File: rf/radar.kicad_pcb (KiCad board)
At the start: 4 copper layers, 52 x 68 mm, 136 parts, among them J101 Conn_01x02, J102 Conn_Coaxial, J103 Conn_01x04, J104 Conn_01x01, J105 Conn_01x01, J106 Conn_Coaxial, J107 Conn_01x02, J108 Conn_01x02, J801 Conn_01x02, T401 2450BL15B100, T402 2450BL15B050, U101 CP0402Q5425ENTR, U201 MAX2750, U202 MC2016K30.0000C16ESH, U203 ADF4153A, U301 QPA5219, U401 AD8343, U501 MGA-645T6, U502 MGA-645T6, U601 TLV4172, U701 SN74LV1T34, U702 SN74LV1T34, U801 ADP150AUJZ-1.8-R7, U802 LM340MPX-5.0/NOPB, U803 L78L33ABU, U804 TPS54308

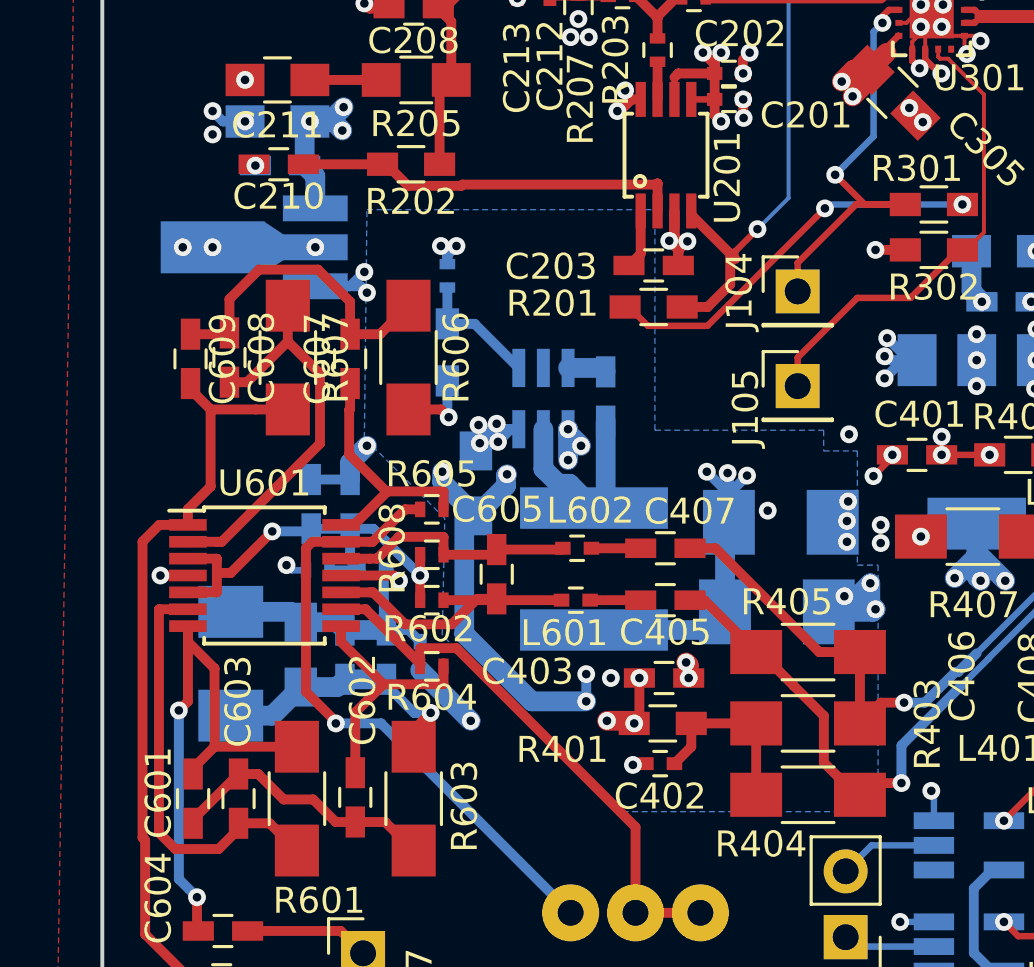
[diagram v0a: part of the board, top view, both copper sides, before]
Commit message: Small fixes; update Gerber
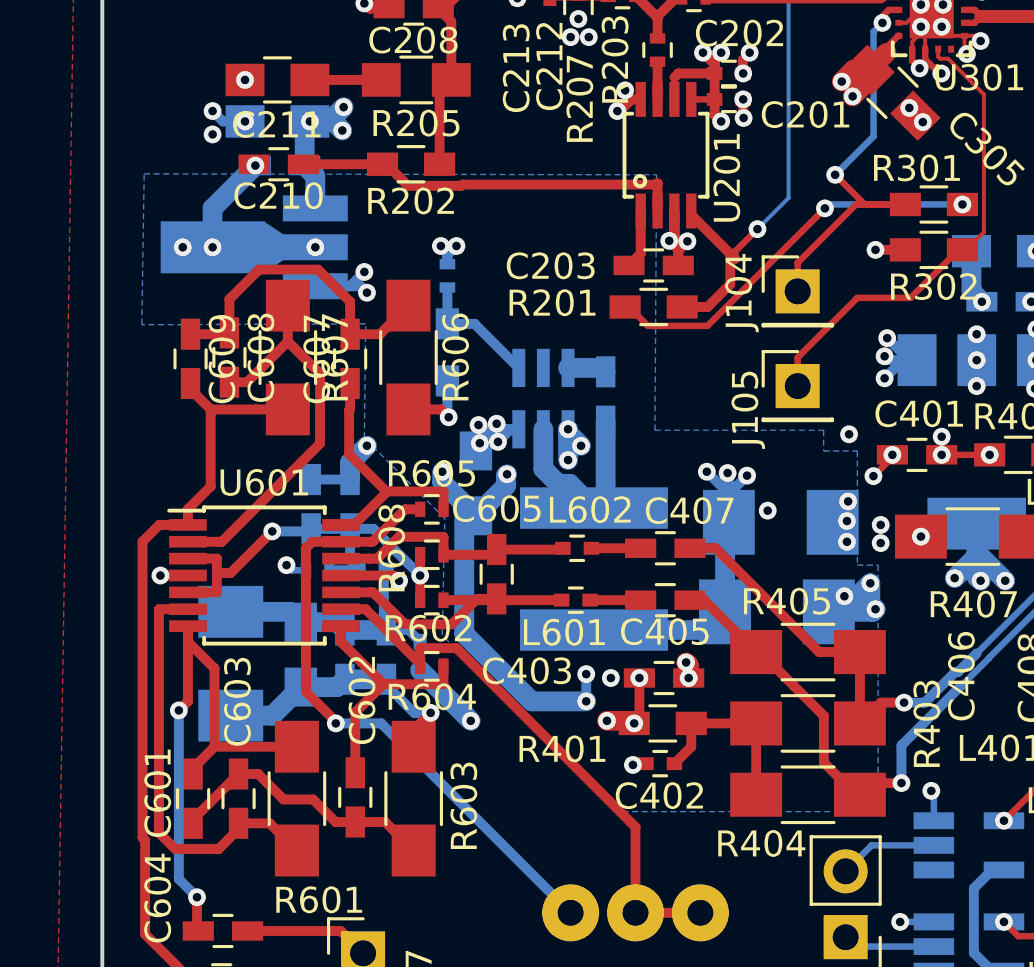
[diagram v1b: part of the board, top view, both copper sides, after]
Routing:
- net GND: track 825.6 -> 839.3 mm
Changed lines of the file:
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@@
     (thickness 1.6)
     (drawings 4)
-    (tracks 1740)
+    (tracks 1741)
     (zones 0)
     (modules 136)
@@
   )
   (setup
-    (last_trace_width 0.1524)
+    (last_trace_width 0.762)
     (user_trace_width 0.25)
     (user_trace_width 0.381)
@@
   (gr_line (start 152 100) (end 152 168) (layer Edge.Cuts) (width 0.15))
   (gr_line (start 100 100) (end 152 100) (layer Edge.Cuts) (width 0.15))
+  (segment (start 104.25 126.25) (end 104.25 124.75) (width 0.762) (layer B.Cu) (net 1))
+  (segment (start 104.25 124.75) (end 105.9 123.1) (width 0.762) (layer B.Cu) (net 1))
+  (segment (start 115.95 132.3) (end 115.95 130.9497) (width 0.762) (layer In2.Cu) (net 1))
+  (segment (start 115.95 130.9497) (end 115.95 130.45) (width 0.762) (layer In2.Cu) (net 1))
+  (segment (start 107.1877 130.9497) (end 115.95 130.9497) (width 0.762) (layer In2.Cu) (net 1))
+  (segment (start 104.25 126.25) (end 104.25 128.012) (width 0.762) (layer In2.Cu) (net 1))
+  (segment (start 104.25 128.012) (end 107.1877 130.9497) (width 0.762) (layer In2.Cu) (net 1))
+  (segment (start 104.25 126.25) (end 108.21 126.25) (width 0.762) (layer In2.Cu) (net 1))
+  (segment (start 103.1 126.25) (end 104.25 126.25) (width 0.762) (layer In2.Cu) (net 1))
   (segment (start 131.715 118.615) (end 131.715 119.0025) (width 0.25) (layer F.Cu) (net 1))
   (segment (start 128.4 129.7) (end 131 127.1) (width 0.762) (layer In1.Cu) (net 1))
@@
   (segment (start 117.95 133.262) (end 118.962 133.262) (width 0.762) (layer In2.Cu) (net 1))
   (segment (start 118.962 133.262) (end 119.35 132.874) (width 0.762) (layer In2.Cu) (net 1))
-  (segment (start 115.95 132.3) (end 115.95 130.45) (width 0.762) (layer In2.Cu) (net 1))
   (segment (start 116.912 133.262) (end 115.95 132.3) (width 0.762) (layer In2.Cu) (net 1))
   (segment (start 116.938 133.262) (end 116.912 133.262) (width 0.762) (layer In2.Cu) (net 1))
@@
   (segment (start 118.35 117.85) (end 118.05 118.15) (width 0.762) (layer In1.Cu) (net 1))
   (segment (start 115.75 112.45) (end 115.75 114.85) (width 0.762) (layer In1.Cu) (net 1))
-  (segment (start 108.21 126.25) (end 108.21 125.41) (width 0.762) (layer In1.Cu) (net 1))
-  (segment (start 108.21 125.41) (end 105.9 123.1) (width 0.762) (layer In1.Cu) (net 1))
-  (segment (start 103.1 126.25) (end 103.442899 125.907101) (width 0.762) (layer In1.Cu) (net 1))
-  (segment (start 103.442899 125.907101) (end 103.442899 125.557101) (width 0.762) (layer In1.Cu) (net 1))
-  (segment (start 103.442899 125.557101) (end 104.25 124.75) (width 0.762) (layer In1.Cu) (net 1))
-  (segment (start 104.25 126.25) (end 104.25 124.75) (width 0.762) (layer In1.Cu) (net 1))
-  (segment (start 104.25 124.75) (end 105.9 123.1) (width 0.762) (layer In1.Cu) (net 1))
   (segment (start 105.625 121.4) (end 106.275 120.75) (width 0.762) (layer In1.Cu) (net 1))
   (segment (start 106.275 120.75) (end 107.15 119.875) (width 0.762) (layer In1.Cu) (net 1))
@@
     (polygon
       (pts
-        (xy 121.3 124.8) (xy 121.3 129) (xy 121.3 133.3) (xy 127.8 133.3) (xy 127.8 134.1)
-        (xy 129.1 134.1) (xy 129.1 138.5) (xy 129.9 138.5) (xy 129.9 141.6) (xy 129.9 144.5)
-        (xy 129.9 148) (xy 119.9 148) (xy 113.1 141.2) (xy 113.2 136.7) (xy 110.1 133.6)
-        (xy 110.2 124.8)
+        (xy 121.3612 123.4567) (xy 121.3 133.3) (xy 127.8 133.3) (xy 127.8 134.1) (xy 129.1 134.1)
+        (xy 129.1 138.5) (xy 129.9 138.5) (xy 129.9 148) (xy 119.9 148) (xy 113.1 141.2)
+        (xy 113.2 136.7) (xy 110.1 133.6) (xy 110.15 129.2) (xy 101.5238 129.2352) (xy 101.6127 123.4186)
       )
     )
@@
         (xy 128.8 140.8) (xy 128.3 140.3) (xy 118 140.3) (xy 118 145) (xy 119 145)
         (xy 119 149) (xy 128 149) (xy 128 168) (xy 100 168) (xy 100 127.2)
-        (xy 128.3 127.2) (xy 128.3 126.7) (xy 100 126.7) (xy 100 100) (xy 152 100)
+        (xy 128.3 127.2) (xy 128.3 126.7) (xy 111.3028 126.7079) (xy 111.3028 125.1839) (xy 99.9998 125.1839)
+        (xy 100 100) (xy 152 100)
       )
     )
